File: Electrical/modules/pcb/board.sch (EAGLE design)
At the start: 108 parts, among them IC1 OP-AMP, IC2 LM311N, IC3 LM311N, IC4 LM311N, IC5 LM311N, IC6 LM311N, M1 SERVO, M2 SERVO, M3 SERVO, U1 QRD1114, U2 LT1161CNPBF, U3 QRD1114, U4 QRD1114, U5 LT1161CNPBF, U6 QRD1114

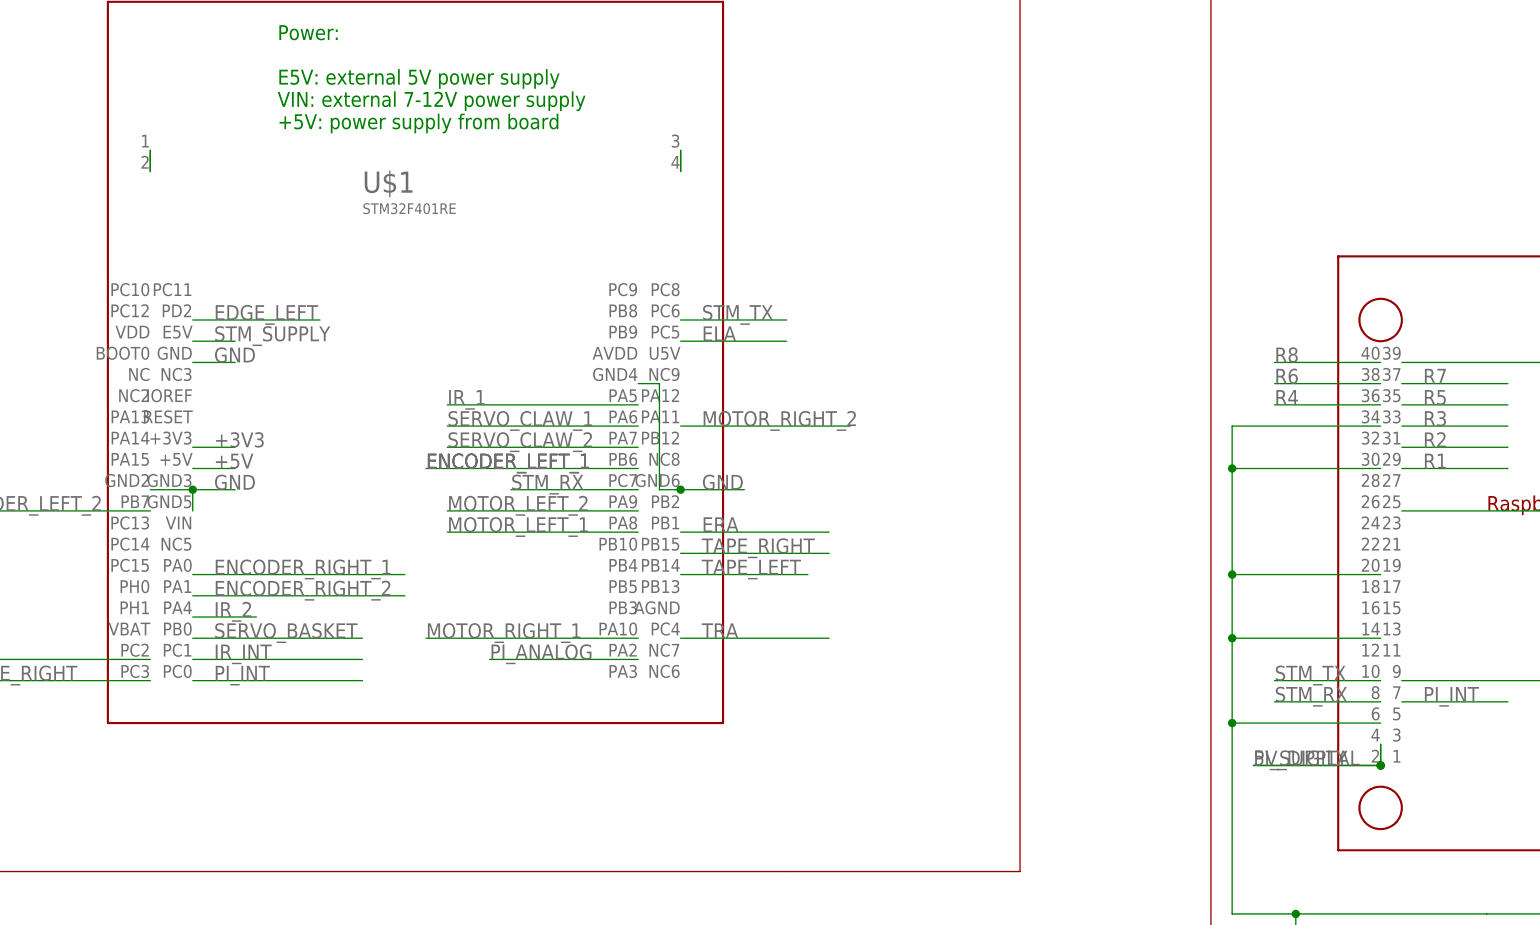
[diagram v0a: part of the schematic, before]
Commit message: fix
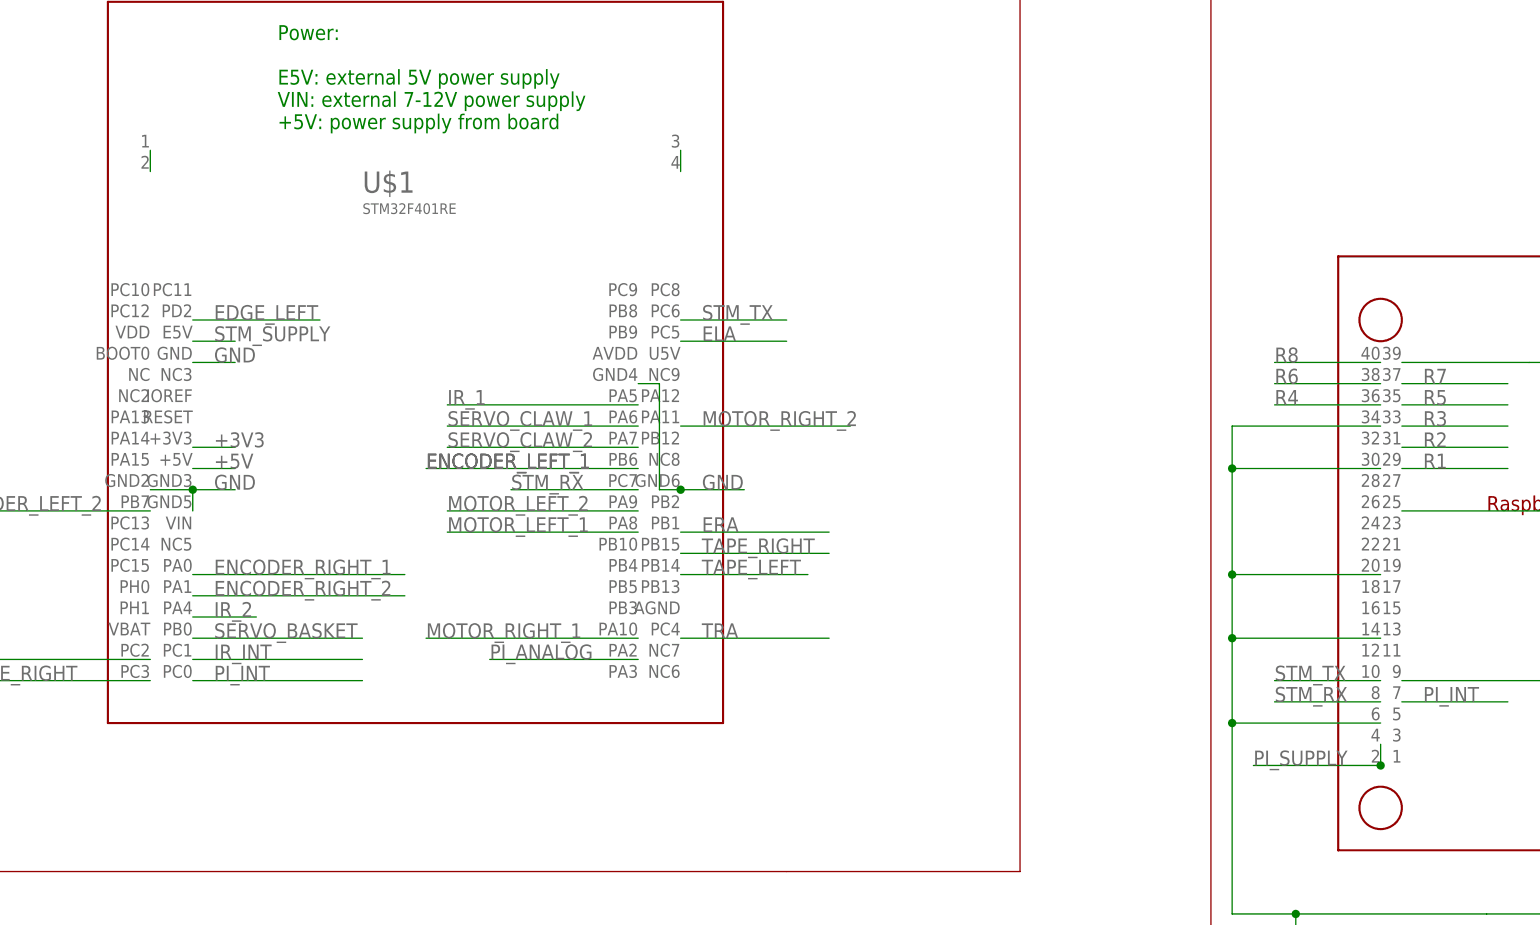
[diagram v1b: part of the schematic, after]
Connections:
- net 5V_DIGITAL: no longer U$6.P$2, U$6.P$4
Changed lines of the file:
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@@
 <junction x="93.98" y="129.54"/>
-</segment>
-<segment>
-<pinref part="U$6" gate="G$1" pin="P$2"/>
-<pinref part="U$6" gate="G$1" pin="P$4"/>
-<wire x1="182.88" y1="208.28" x2="182.88" y2="210.82" width="0.1524" layer="91"/>
-<wire x1="182.88" y1="208.28" x2="167.64" y2="208.28" width="0.1524" layer="91"/>
-<junction x="182.88" y="208.28"/>
-<label x="167.64" y="208.28" size="1.778" layer="95"/>
 </segment>
 </net>
@@
 </segment>
 </net>
-<net name="N$32" class="0">
-<segment>
-<pinref part="U$1" gate="A" pin="P$105"/>
-<pinref part="U$1" gate="A" pin="P$106"/>
-<wire x1="35.56" y1="279.4" x2="35.56" y2="281.94" width="0.1524" layer="91"/>
-</segment>
-</net>
-<net name="N$37" class="0">
-<segment>
-<pinref part="U$1" gate="A" pin="P$108"/>
-<pinref part="U$1" gate="A" pin="P$107"/>
-<wire x1="99.06" y1="279.4" x2="99.06" y2="281.94" width="0.1524" layer="91"/>
-</segment>
-</net>
